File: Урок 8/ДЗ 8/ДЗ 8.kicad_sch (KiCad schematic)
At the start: 23 parts, among them K2 HONGFA_HFD2-0xx-x-L2-x, K3 HONGFA_HFD2-0xx-x-L2-x, SW3 SW_Push, SW4 SW_Push

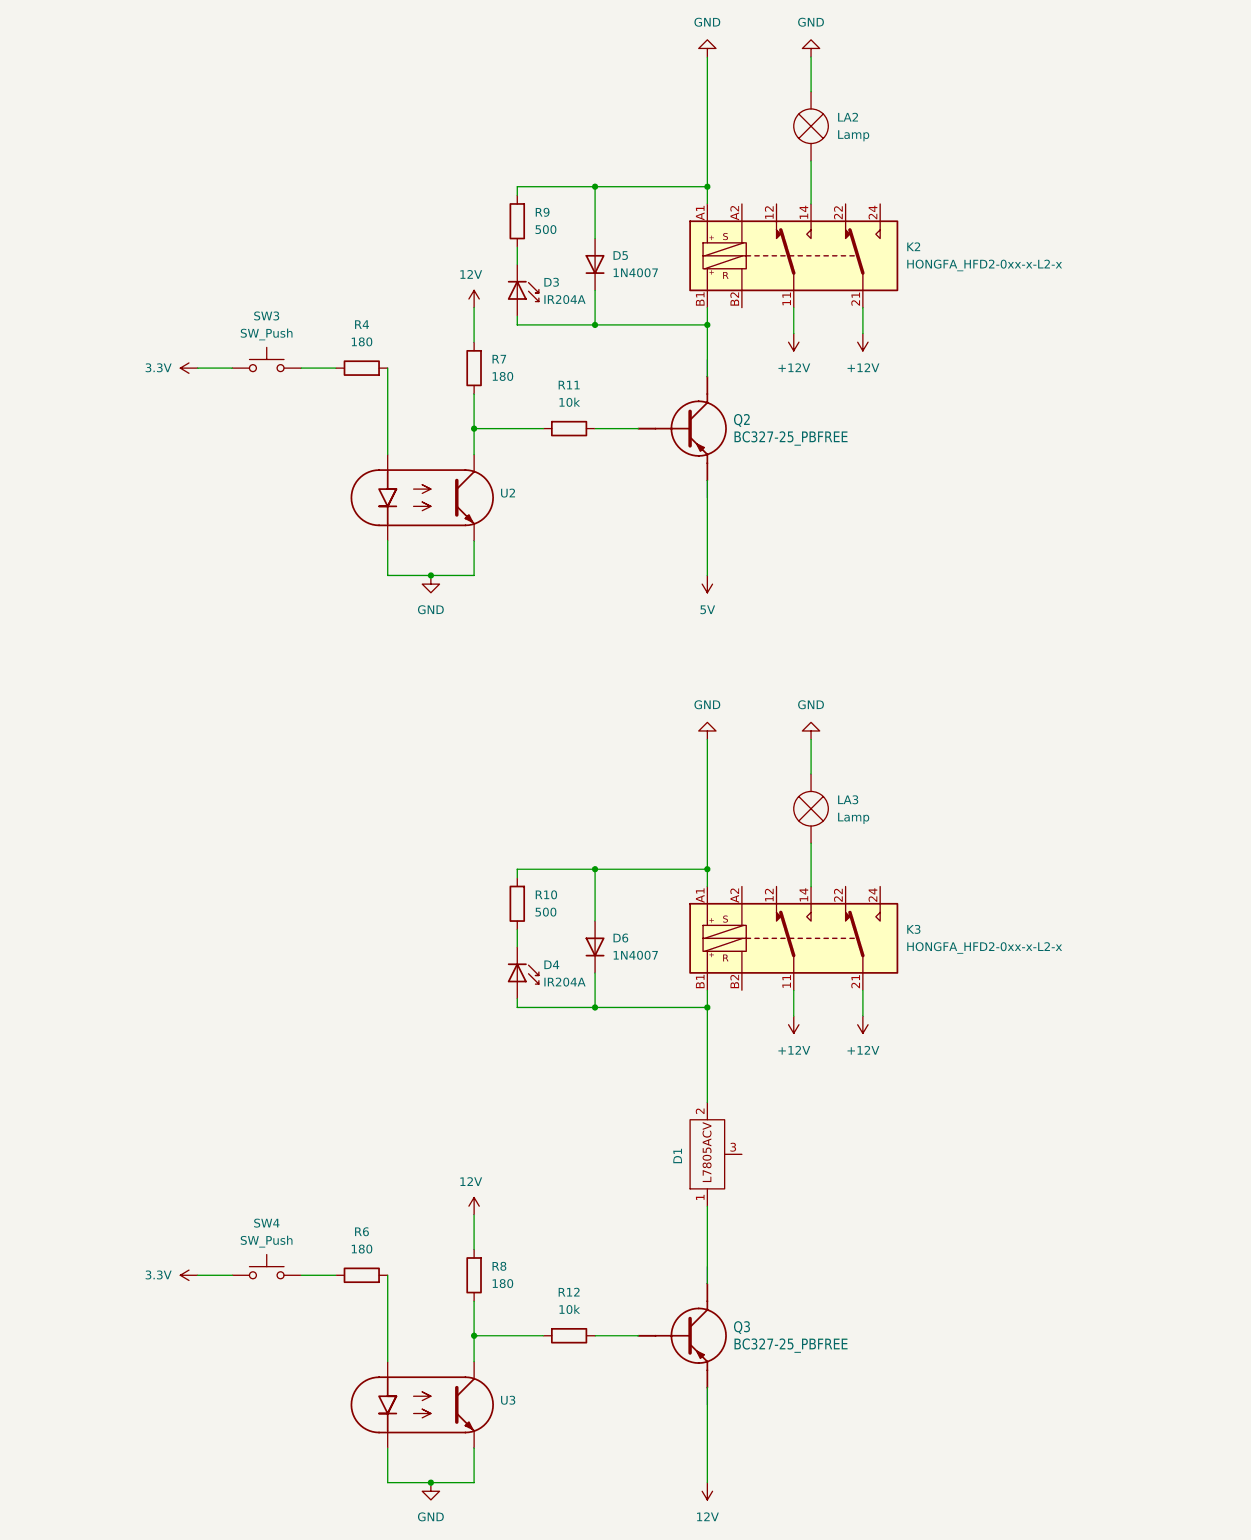
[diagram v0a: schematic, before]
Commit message: 1
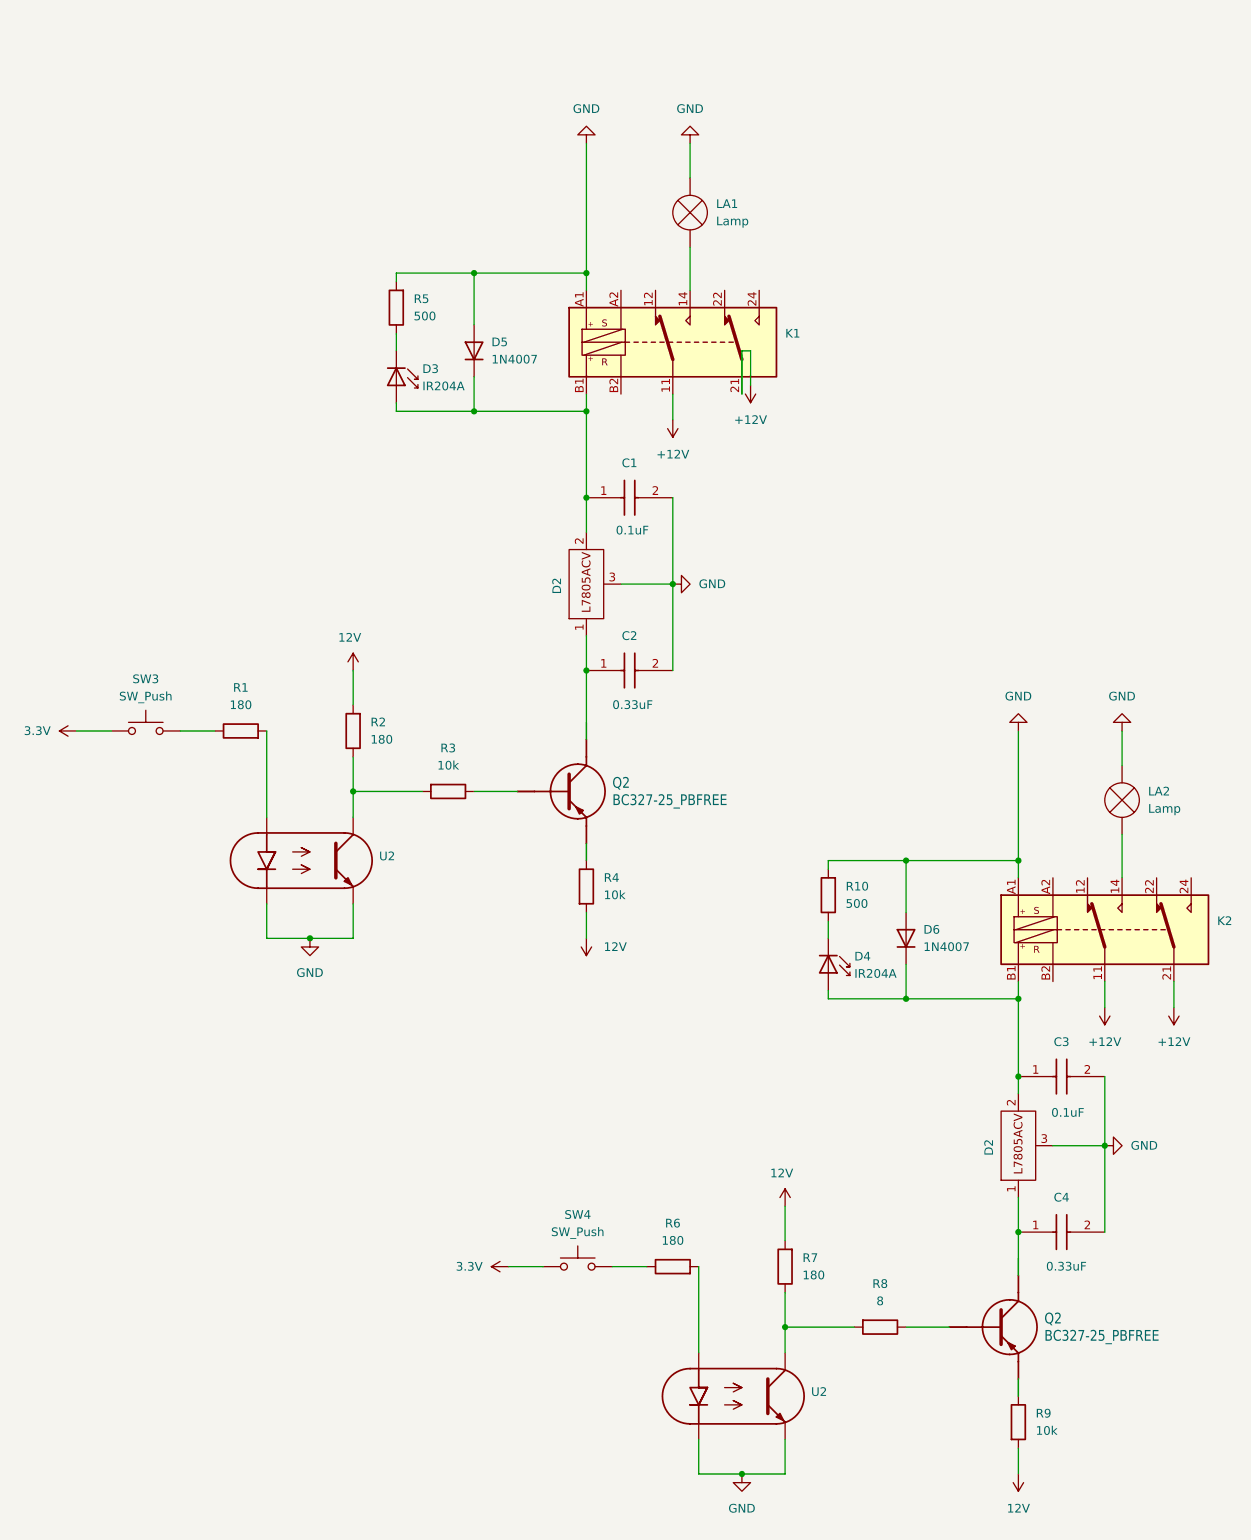
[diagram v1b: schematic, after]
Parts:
- added C1: 0.1uF, My_lib2:564R60GAD10, symbol My_lib2:564R60GAD10
- added C2: 0.33uF, 564R60GAD10, symbol My_lib2:564R60GAD10
- added C3: 0.1uF, 564R60GAD10, symbol My_lib2:564R60GAD10
- added C4: 0.33uF, My_lib2:564R60GAD10, symbol My_lib2:564R60GAD10
- added D2: ~, My_lib2:TO-220 - L7805ACV, symbol My_lib2:L7805ACV
- added R4, R9: 10k, symbol Device:R
- R8: renamed from R12; value 10k -> 8
- renumbered D1 to D2, K2 to K1, K3 to K2, LA2 to LA1, LA3 to LA2, Q3 to Q2, R4 to R1, R7 to R2, R11 to R3, R9 to R5, R8 to R7, U3 to U2
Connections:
- net 12V: now also R4.2, R9.2; no longer Q2.3 (A)
- net GND: now also D2.3 (GND), C1.2, C2.2, C3.2, C4.2, D2.3 (GND)
- net at D2.1, Q2.1 (C): now also C4.1
- net at D2.2, D4.2 (A), D6.1 (K)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: now also C3.1
- net at D3.2 (A), D5.1 (K), K1.B1: now also C1.1, D2.2; no longer Q2.1 (C)
- net 5V: no longer names the net of Q2.3 (A)
- net 5V: now also R4.1
- new net: C2.1, D2.1, Q2.1 (C)
- new net: Q2.3 (A), R9.1
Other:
- moved on the sheet: D2, D3, D4, D5, D6, K1, K2, LA1, LA2, Q2, R1, R10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

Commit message: 1
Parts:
- removed SW3, SW4: SW_Push, symbol Switch:SW_Push
- added SW1, SW2: SW_Push, My_lib2:0650HIM-130G-G, symbol My_lib2:SW_Push
- C1, C4: footprint My_lib2:564R60GAD10 -> 564R60GAD10
- U2: footprint (none) -> My_lib2:DIP762W60P254L460H450Q4N
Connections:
- net 3.3V: now also SW1.1, SW2.1
- net at R1.1: now also SW1.2
- net at R6.1: now also SW2.2
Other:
- moved on the sheet: C1, C2, C3, C4, D2, D3, D4, D5, D6, K1, K2, LA1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
